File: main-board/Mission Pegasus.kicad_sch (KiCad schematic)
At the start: 15 parts, among them J1 TC2030, J3 FTSH-105-04-L-D-RA, J4 FTSH-105-04-L-D-RA, J5 FTSH-105-04-L-D-RA, Q1 DTC113Z

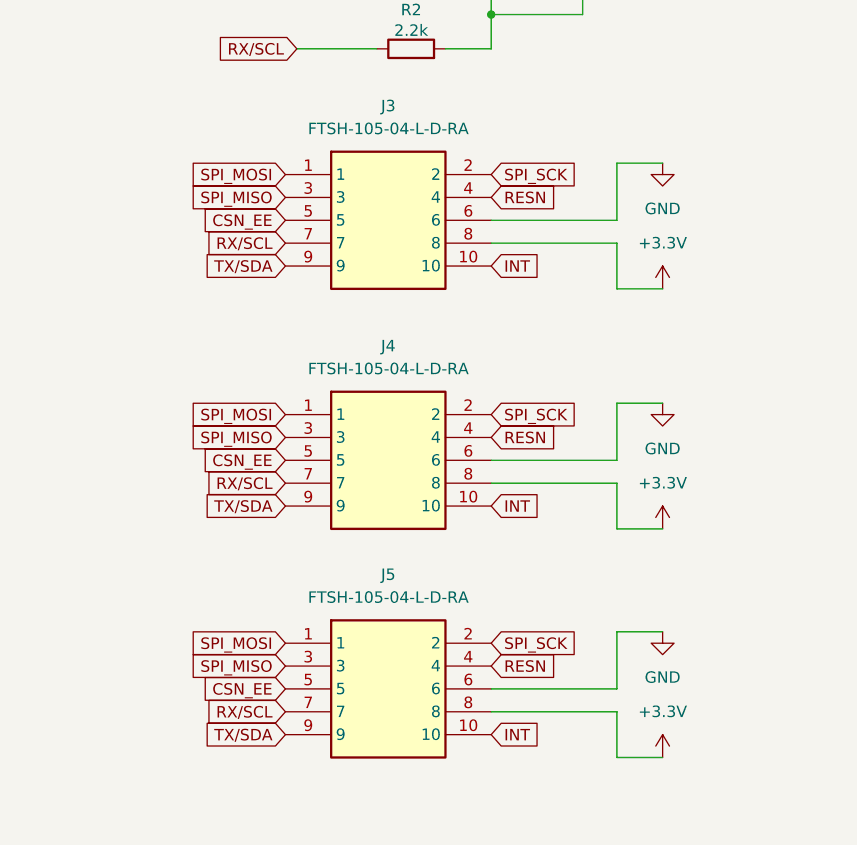
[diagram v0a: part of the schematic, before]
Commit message: Update larger board design
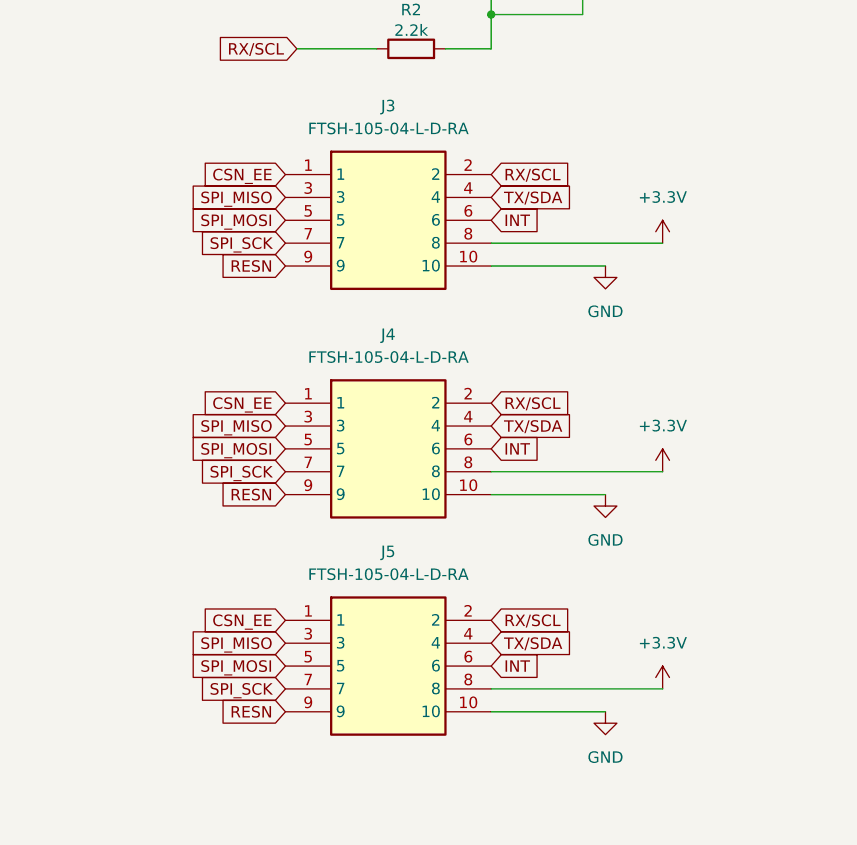
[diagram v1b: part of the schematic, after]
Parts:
- H3, H4, H5, H6, H7, H8: footprint Mounting_Wuerth:Mounting_Wuerth_WA-SMSI-M2.5_H0.5mm_9774005151 -> MountingHole:MountingHole_2.7mm_M2.5
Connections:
- net CSN_EE: now also J3.1, J4.1, J5.1; no longer J3.5, J4.5, J5.5
- net GND: now also J3.10, J4.10, J5.10; no longer J3.6, J4.6, J5.6
- net INT: now also J3.6, J4.6, J5.6; no longer J3.10, J4.10, J5.10
- net RESN: now also J3.9, J4.9, J5.9; no longer J3.4, J4.4, J5.4
- net RX/SCL: now also J3.2, J4.2, J5.2; no longer J3.7, J4.7, J5.7
- net SPI_MOSI: now also J3.5, J4.5, J5.5; no longer J3.1, J4.1, J5.1
- net SPI_SCK: now also J3.7, J4.7, J5.7; no longer J3.2, J4.2, J5.2
- net TX/SDA: now also J3.4, J4.4, J5.4; no longer J3.9, J4.9, J5.9
